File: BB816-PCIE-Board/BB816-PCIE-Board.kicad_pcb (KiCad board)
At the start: 4 copper layers, 167.6 x 111.2 mm, 1 part, among them J1 BB816_BreakoutA27_PCIex16

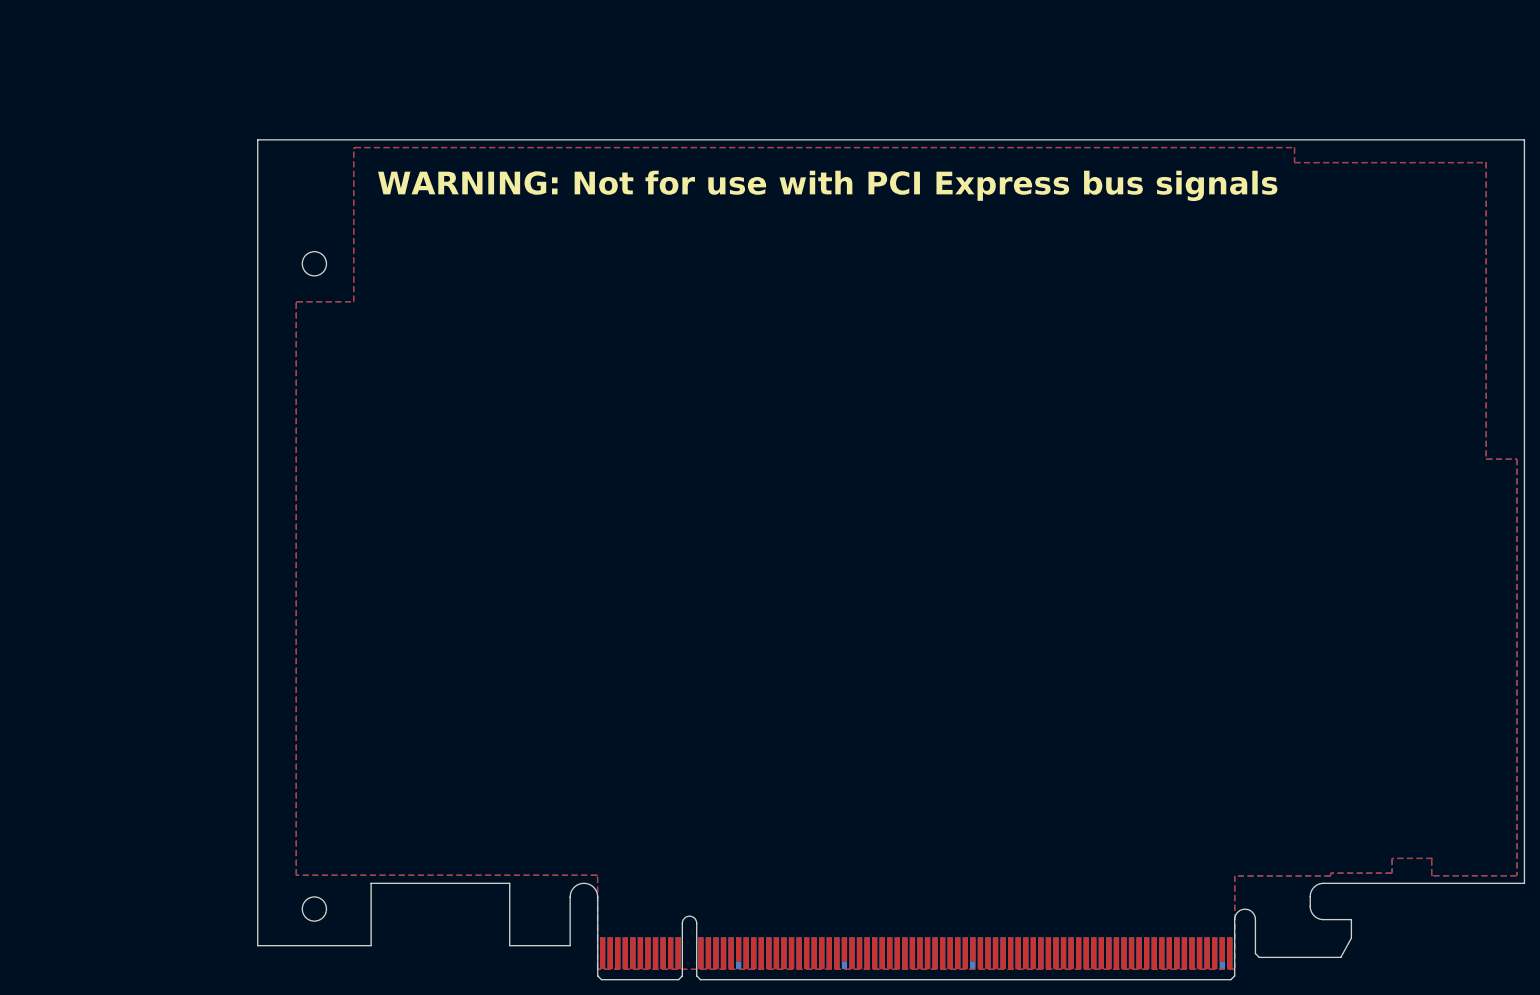
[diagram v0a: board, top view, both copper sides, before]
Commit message: Stuff
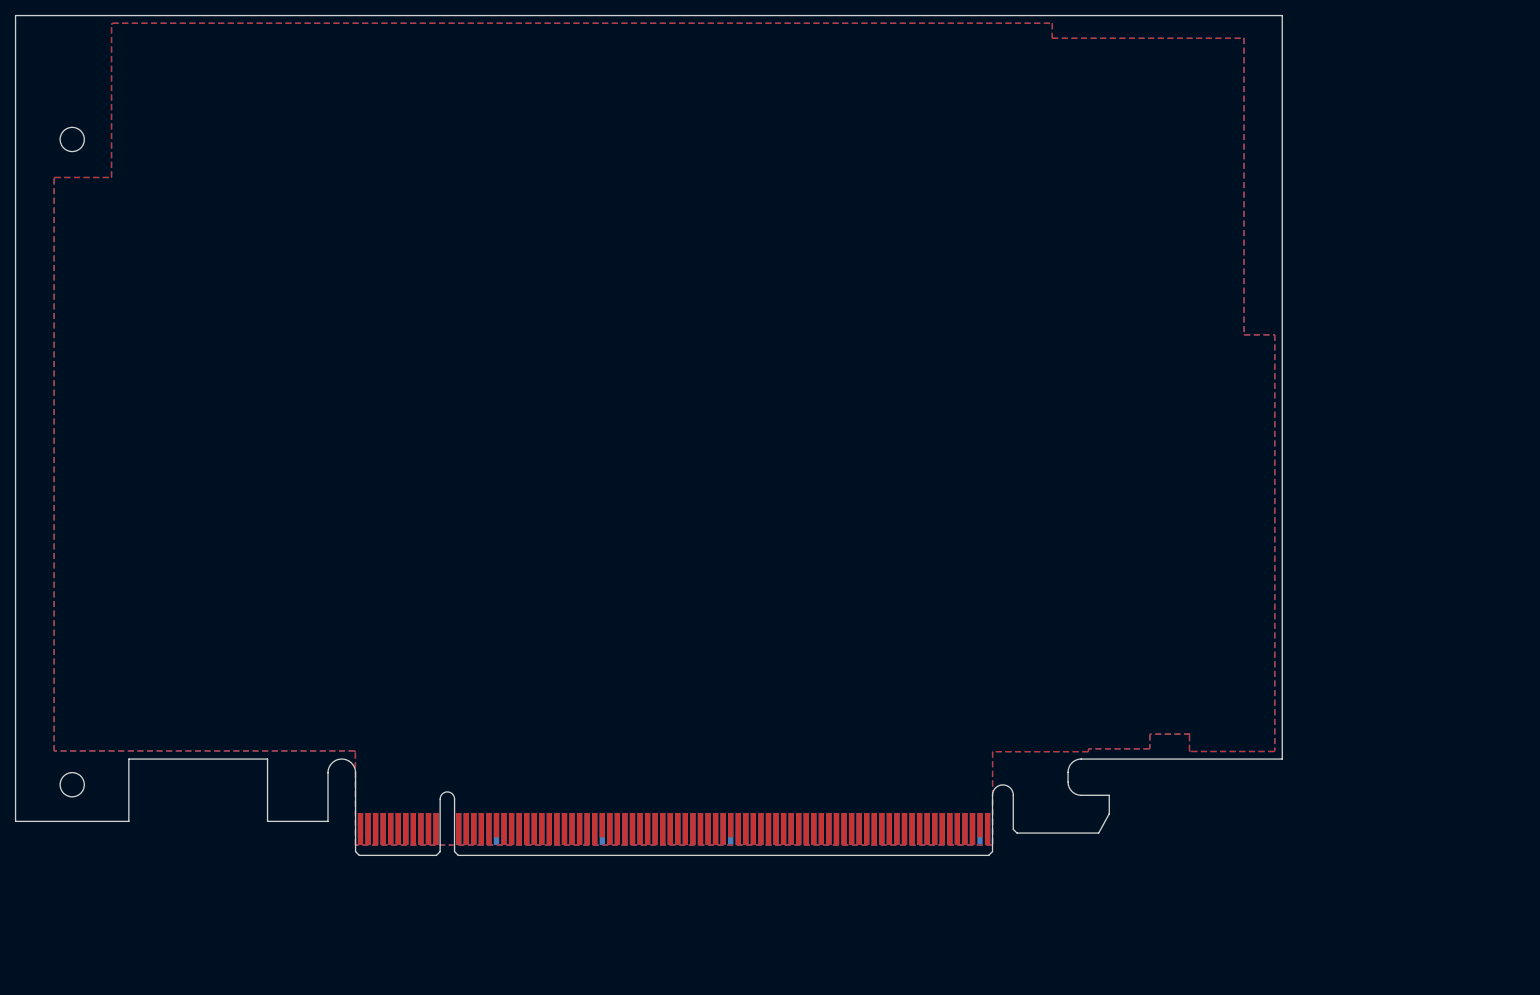
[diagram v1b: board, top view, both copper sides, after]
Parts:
- moved J1 36.0 mm to (70.5, 136.6)
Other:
- board size 167.6 x 111.2 mm -> 167.7 x 111.2 mm
- board text removed: "WARNING: Not for use with PCI Express bus signals"
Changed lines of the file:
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@@
 	(footprint "BB816-MATX-PCIE:PCIexpress_x16_HW_FH"
 		(layer "F.Cu")
-		(at 102.6 153)
+		(at 70.55 136.55)
 		(descr "PCIexpress x16 footprint")
 		(tags "PCIexpress")
@@
 		)
 	)
-	(gr_text "WARNING: Not for use with PCI Express bus signals"
-		(at 73.25 49.43 0)
-		(layer "F.SilkS")
-		(effects
-			(font
-				(size 3 3)
-				(thickness 0.3)
-				(bold yes)
-			)
-			(justify left bottom)
-		)
-	)
 	(zone
 		(net 0)
@@
 		(polygon
 			(pts
-				(xy 70.3 42.87) (xy 194.67 42.87) (xy 194.67 44.84) (xy 194.65 44.86) (xy 220.01 44.86) (xy 220.04 44.83)
-				(xy 220.04 84.08) (xy 220.07 84.11) (xy 224.11 84.11) (xy 224.11 139.16) (xy 224.02 139.25) (xy 212.91 139.25)
-				(xy 212.82 139.16) (xy 212.82 137.02) (xy 212.89 136.95) (xy 207.64 136.95) (xy 207.58 137.01) (xy 207.58 138.83)
-				(xy 207.51 138.9) (xy 199.5 138.9) (xy 199.45 138.95) (xy 199.45 139.24) (xy 199.42 139.27) (xy 186.76 139.27)
-				(xy 186.76 151.6) (xy 186.73 151.63) (xy 102.43 151.63) (xy 102.43 139.29) (xy 102.32 139.18) (xy 62.55 139.18)
-				(xy 62.55 63.37) (xy 62.64 63.28) (xy 70.14 63.28) (xy 70.15 63.27) (xy 70.15 43.02)
+				(xy 38.25 26.42) (xy 162.62 26.42) (xy 162.62 28.39) (xy 162.6 28.41) (xy 187.96 28.41) (xy 187.99 28.38)
+				(xy 187.99 67.63) (xy 188.02 67.66) (xy 192.06 67.66) (xy 192.06 122.71) (xy 191.97 122.8) (xy 180.86 122.8)
+				(xy 180.77 122.71) (xy 180.77 120.57) (xy 180.84 120.5) (xy 175.59 120.5) (xy 175.53 120.56) (xy 175.53 122.38)
+				(xy 175.46 122.45) (xy 167.45 122.45) (xy 167.4 122.5) (xy 167.4 122.79) (xy 167.37 122.82) (xy 154.71 122.82)
+				(xy 154.71 135.15) (xy 154.68 135.18) (xy 70.38 135.18) (xy 70.38 122.84) (xy 70.27 122.73) (xy 30.5 122.73)
+				(xy 30.5 46.92) (xy 30.59 46.83) (xy 38.09 46.83) (xy 38.1 46.82) (xy 38.1 26.57)
 			)
 		)
@@
 		(polygon
 			(pts
-				(xy 70.17 42.79) (xy 194.54 42.79) (xy 194.54 44.76) (xy 194.52 44.78) (xy 219.88 44.78) (xy 219.91 44.75)
-				(xy 219.91 84) (xy 219.94 84.03) (xy 223.98 84.03) (xy 223.98 139.08) (xy 223.89 139.17) (xy 212.78 139.17)
-				(xy 212.69 139.08) (xy 212.69 136.94) (xy 212.76 136.87) (xy 207.51 136.87) (xy 207.45 136.93) (xy 207.45 138.75)
-				(xy 207.38 138.82) (xy 199.37 138.82) (xy 199.32 138.87) (xy 199.32 139.16) (xy 199.29 139.19) (xy 186.63 139.19)
-				(xy 186.63 151.52) (xy 186.6 151.55) (xy 102.3 151.55) (xy 102.3 139.21) (xy 102.19 139.1) (xy 62.42 139.1)
-				(xy 62.42 63.29) (xy 62.51 63.2) (xy 70.01 63.2) (xy 70.02 63.19) (xy 70.02 42.94)
+				(xy 38.12 26.34) (xy 162.49 26.34) (xy 162.49 28.31) (xy 162.47 28.33) (xy 187.83 28.33) (xy 187.86 28.3)
+				(xy 187.86 67.55) (xy 187.89 67.58) (xy 191.93 67.58) (xy 191.93 122.63) (xy 191.84 122.72) (xy 180.73 122.72)
+				(xy 180.64 122.63) (xy 180.64 120.49) (xy 180.71 120.42) (xy 175.46 120.42) (xy 175.4 120.48) (xy 175.4 122.3)
+				(xy 175.33 122.37) (xy 167.32 122.37) (xy 167.27 122.42) (xy 167.27 122.71) (xy 167.24 122.74) (xy 154.58 122.74)
+				(xy 154.58 135.07) (xy 154.55 135.1) (xy 70.25 135.1) (xy 70.25 122.76) (xy 70.14 122.65) (xy 30.37 122.65)
+				(xy 30.37 46.84) (xy 30.46 46.75) (xy 37.96 46.75) (xy 37.97 46.74) (xy 37.97 26.49)
 			)
 		)
 	)
+	(group ""
+		(members "2764cc48-0fdd-4b5f-a986-97a4fdcc3559" "de5eaf54-25bf-40eb-9686-d723e0ac6e9d"
+			"e348be87-3b3e-4da6-88e7-7739e6966a6b"
+		)
+	)
